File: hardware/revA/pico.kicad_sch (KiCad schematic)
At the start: 8 parts, among them Q20 MMBT4401-7-F, Q21 IRF7404TRPBF, U25 Pico

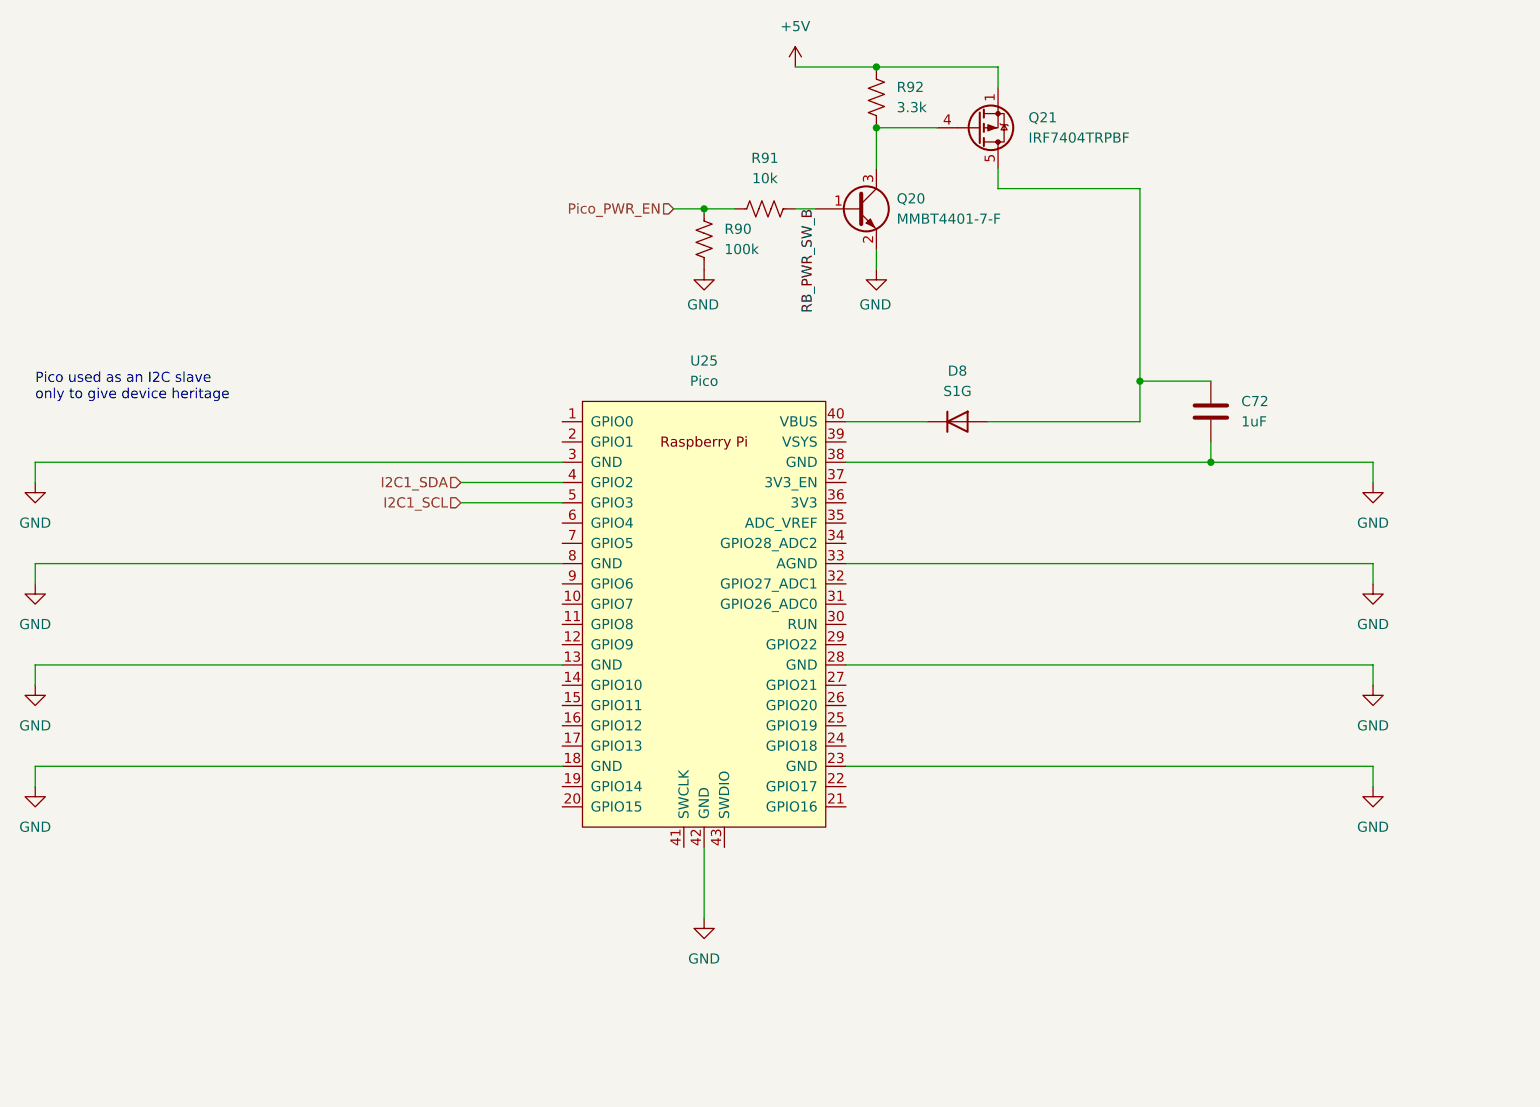
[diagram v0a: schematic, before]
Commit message: working revB
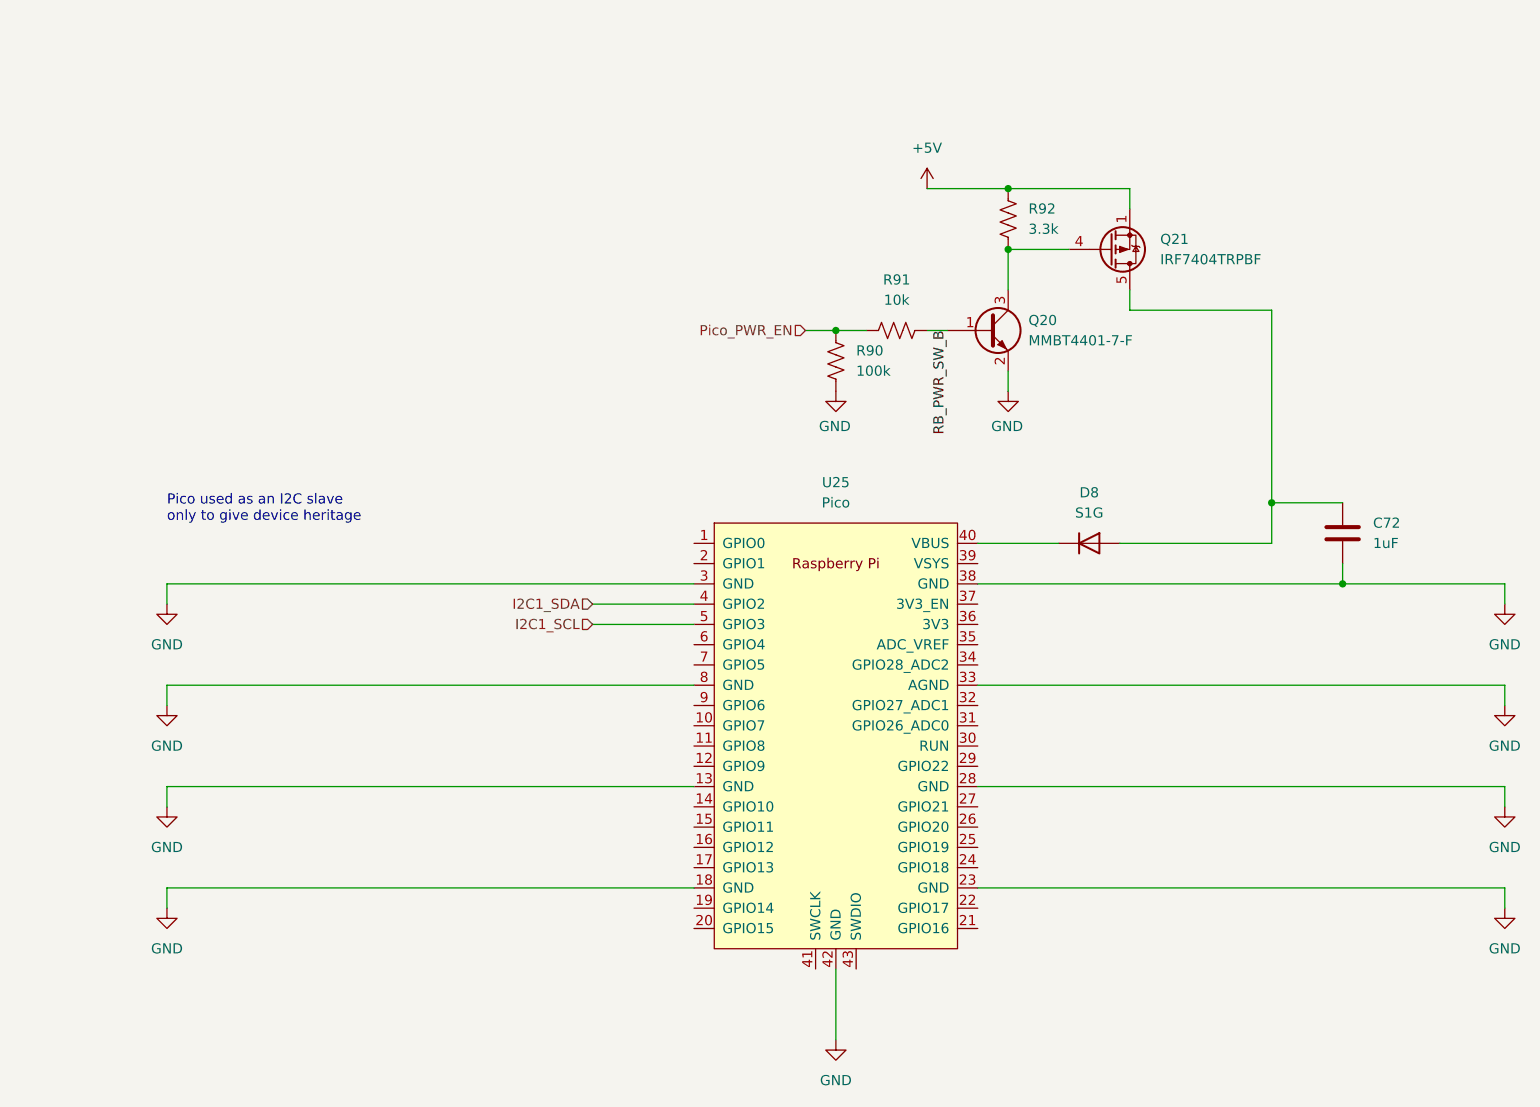
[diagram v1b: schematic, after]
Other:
- company: (none) -> Sierra Lobo INC
- moved on the sheet: C72, D8, Q20, Q21, R90, R91, R92, U25
